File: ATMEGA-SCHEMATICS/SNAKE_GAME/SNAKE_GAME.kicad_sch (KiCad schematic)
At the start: 7 parts

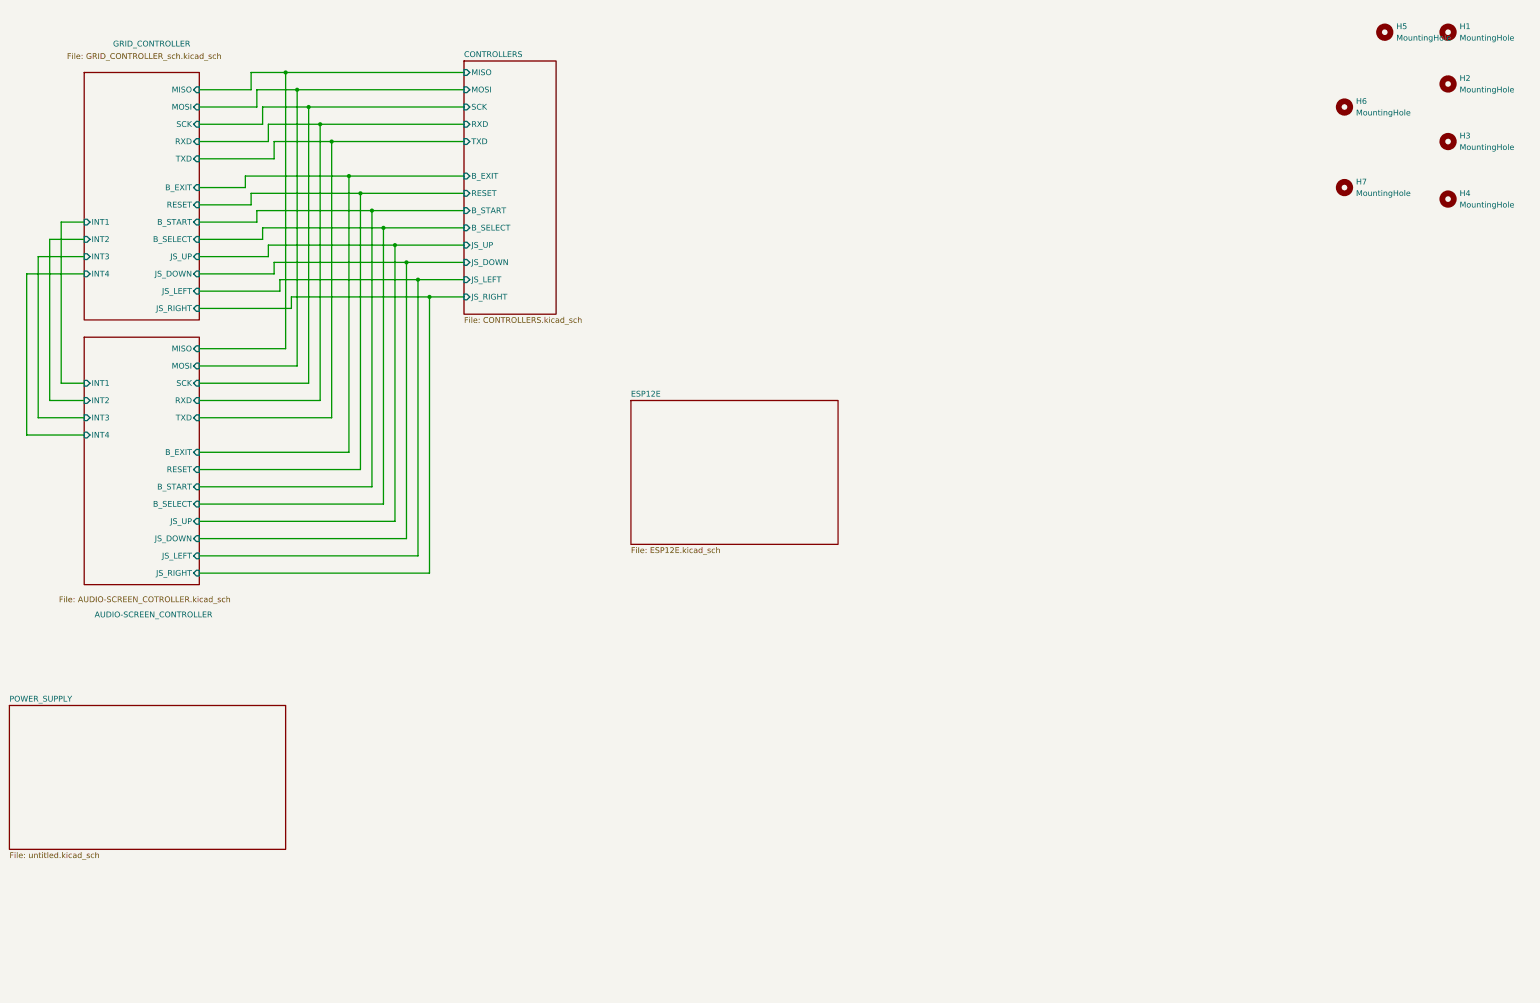
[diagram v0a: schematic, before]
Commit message: .
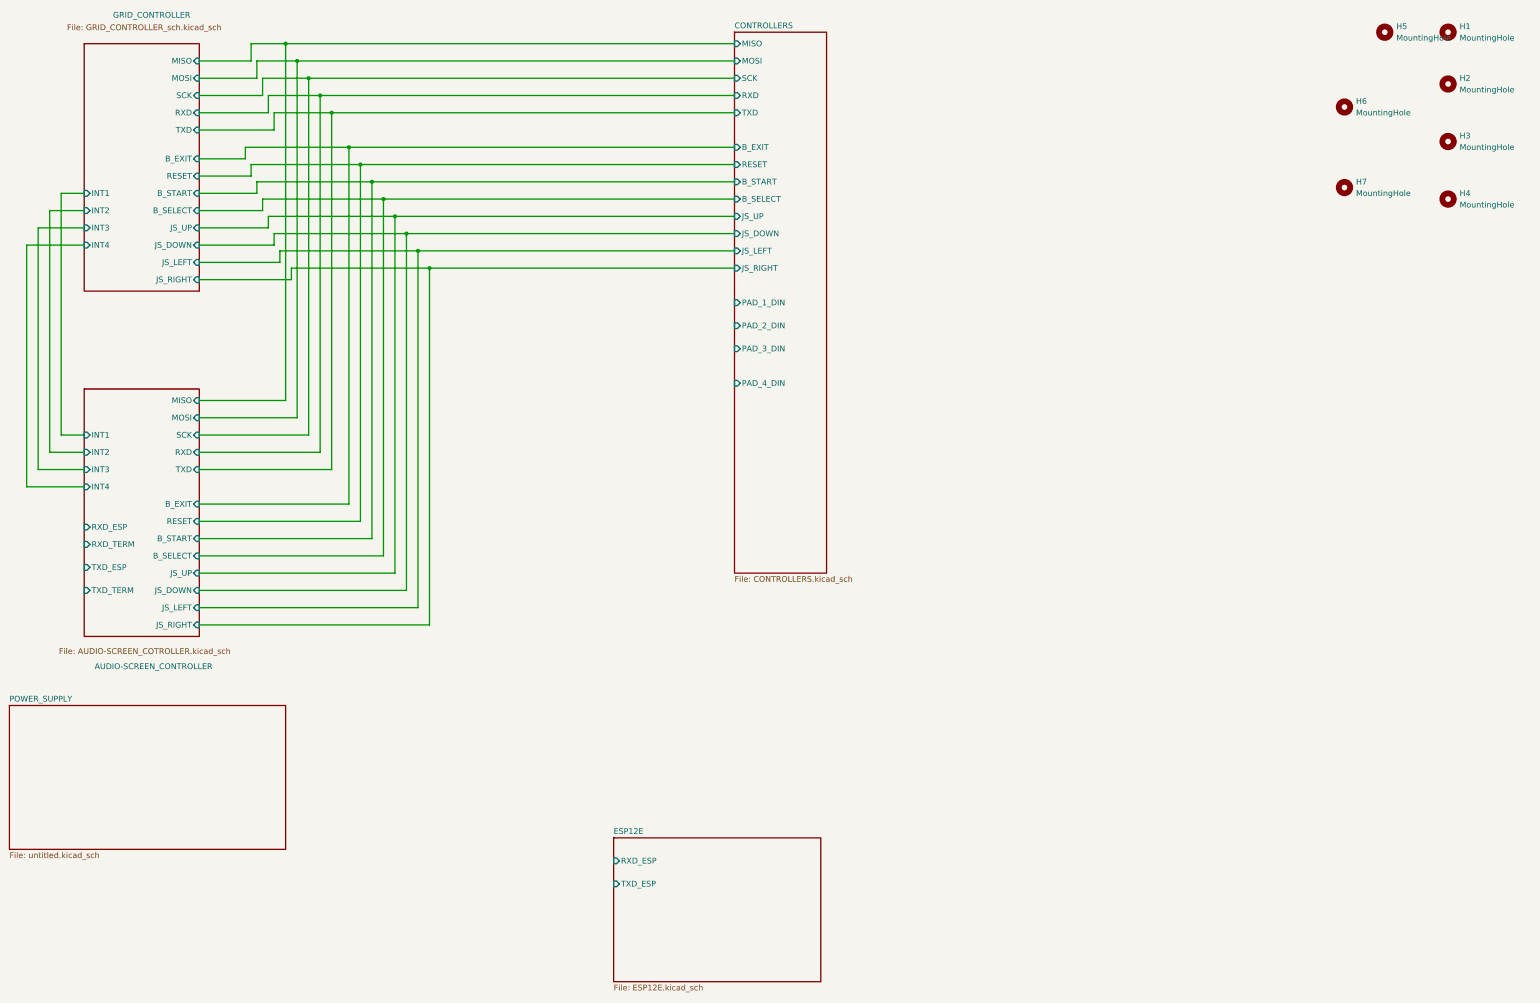
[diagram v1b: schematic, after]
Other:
- sheet AUDIO-SCREEN_CONTROLLER ports: added RXD_ESP, RXD_TERM, TXD_ESP, TXD_TERM; removed none
- sheet CONTROLLERS ports: added PAD_1_DIN, PAD_2_DIN, PAD_3_DIN, PAD_4_DIN; removed none
- sheet ESP12E ports: added RXD_ESP, TXD_ESP; removed none
